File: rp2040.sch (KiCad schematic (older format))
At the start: 29 parts, among them Q5 Q_NMOS_GSD, U17 W25Q128JVS, U3 RP2040, Y2 12MHz

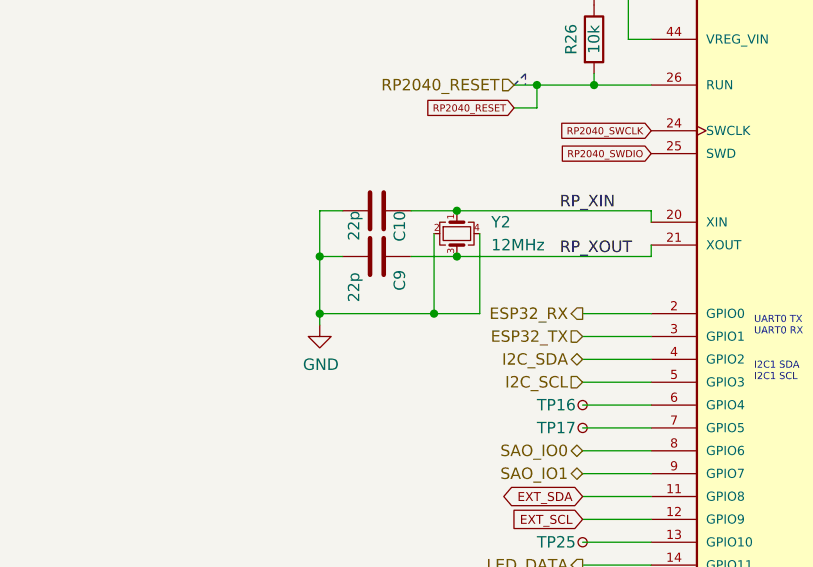
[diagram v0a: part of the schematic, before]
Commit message: Add 1k resistor for RP2040 crystal, add schematic PDF
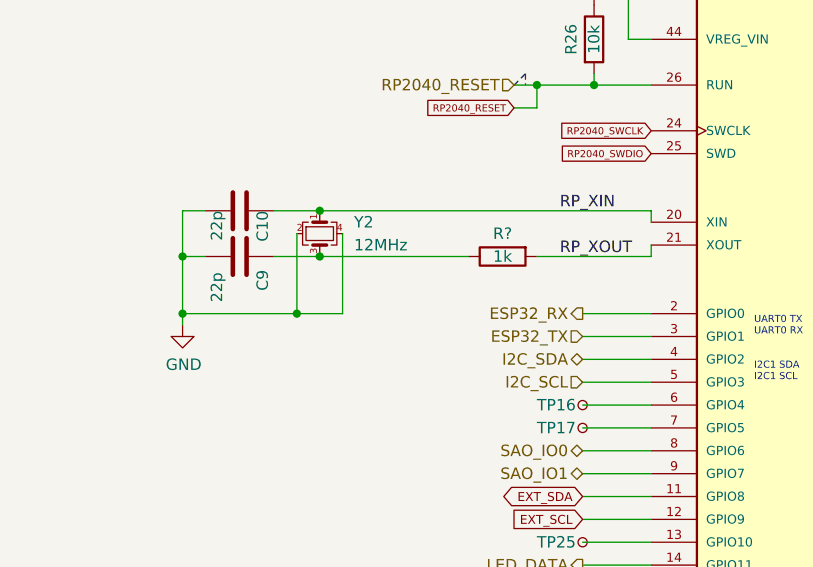
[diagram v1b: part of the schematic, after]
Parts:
- added R?: 1k, Resistor_SMD:R_0402_1005Metric, symbol mch2021-rescue:R-Device
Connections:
- net RP_XOUT: now also R?.2; no longer C9.1, Y2.3
- new net: C9.1, R?.1, Y2.3
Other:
- moved on the sheet: C10, C9, Y2
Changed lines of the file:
@@
 encoding utf-8
 Sheet 3 9
-Title "MCH2021 badge - RP2040 microcontroller"
-Date "2021-11-14"
-Rev "3"
+Title "MCH2022 badge - RP2040 microcontroller"
+Date "2021-12-19"
+Rev "3.1415"
 Comp "BADGE.TEAM"
 Comment1 ""
@@
 L mch2021-rescue:C-Device C?
 U 1 1 5E3EFF6B
-P 3100 3200
+P 2500 3200
 AR Path="/5DC753C3/5E3EFF6B" Ref="C?"  Part="1"
 AR Path="/5E3EFF6B" Ref="C?"  Part="1"
 AR Path="/5E3BA64A/5E3EFF6B" Ref="C?"  Part="1"
 AR Path="/5F51E414/5E3EFF6B" Ref="C10"  Part="1"
-F 0 "C10" H 3100 3300 50  0000 L CNN
-F 1 "22p" H 3100 3100 50  0000 L CNN
-F 2 "Capacitor_SMD:C_0402_1005Metric" H 3138 3050 50  0001 C CNN
-F 3 "" H 3100 3200 50  0001 C CNN
-F 4 "C696906" H 3100 3200 50  0001 C CNN "LCSC"
-F 5 "" H 3100 3200 50  0001 C CNN "Price"
-F 6 "N" H 3100 3200 50  0001 C CNN "Sponsored"
-	1    3100 3200
+F 0 "C10" H 2500 3300 50  0000 L CNN
+F 1 "22p" H 2500 3100 50  0000 L CNN
+F 2 "Capacitor_SMD:C_0402_1005Metric" H 2538 3050 50  0001 C CNN
+F 3 "" H 2500 3200 50  0001 C CNN
+F 4 "C696906" H 2500 3200 50  0001 C CNN "LCSC"
+F 5 "" H 2500 3200 50  0001 C CNN "Price"
+F 6 "N" H 2500 3200 50  0001 C CNN "Sponsored"
+	1    2500 3200
 	0    1    1    0
 $EndComp
@@
 L mch2021-rescue:C-Device C?
 U 1 1 5E3F1F93
-P 3100 3400
+P 2500 3400
 AR Path="/5DC753C3/5E3F1F93" Ref="C?"  Part="1"
 AR Path="/5E3F1F93" Ref="C?"  Part="1"
 AR Path="/5E3BA64A/5E3F1F93" Ref="C?"  Part="1"
 AR Path="/5F51E414/5E3F1F93" Ref="C9"  Part="1"
-F 0 "C9" H 2950 3500 50  0000 L CNN
-F 1 "22p" H 2900 3300 50  0000 L CNN
-F 2 "Capacitor_SMD:C_0402_1005Metric" H 3138 3250 50  0001 C CNN
-F 3 "" H 3100 3400 50  0001 C CNN
-F 4 "C696906" H 3100 3400 50  0001 C CNN "LCSC"
-F 5 "" H 3100 3400 50  0001 C CNN "Price"
-F 6 "N" H 3100 3400 50  0001 C CNN "Sponsored"
-	1    3100 3400
+F 0 "C9" H 2350 3500 50  0000 L CNN
+F 1 "22p" H 2300 3300 50  0000 L CNN
+F 2 "Capacitor_SMD:C_0402_1005Metric" H 2538 3250 50  0001 C CNN
+F 3 "" H 2500 3400 50  0001 C CNN
+F 4 "C696906" H 2500 3400 50  0001 C CNN "LCSC"
+F 5 "" H 2500 3400 50  0001 C CNN "Price"
+F 6 "N" H 2500 3400 50  0001 C CNN "Sponsored"
+	1    2500 3400
 	0    1    -1   0
 $EndComp
@@
 L mch2021-rescue:Crystal_GND24_Small-Device Y2
 U 1 1 5E3ED918
-P 3450 3300
-F 0 "Y2" V 3400 3450 50  0000 L CNN
-F 1 "12MHz" V 3500 3450 50  0000 L CNN
-F 2 "Crystal:Crystal_SMD_3225-4Pin_3.2x2.5mm" H 3450 3300 50  0001 C CNN
-F 3 "~" H 3450 3300 50  0001 C CNN
-F 4 "C13738" H 3450 3300 50  0001 C CNN "LCSC"
-F 5 "" H 3450 3300 50  0001 C CNN "Price"
-F 6 "-" H 3450 3300 50  0001 C CNN "Mouser"
-F 7 "N" H 3450 3300 50  0001 C CNN "Sponsored"
-	1    3450 3300
+P 2850 3300
+F 0 "Y2" V 2800 3450 50  0000 L CNN
+F 1 "12MHz" V 2900 3450 50  0000 L CNN
+F 2 "Crystal:Crystal_SMD_3225-4Pin_3.2x2.5mm" H 2850 3300 50  0001 C CNN
+F 3 "~" H 2850 3300 50  0001 C CNN
+F 4 "C13738" H 2850 3300 50  0001 C CNN "LCSC"
+F 5 "" H 2850 3300 50  0001 C CNN "Price"
+F 6 "-" H 2850 3300 50  0001 C CNN "Mouser"
+F 7 "N" H 2850 3300 50  0001 C CNN "Sponsored"
+	1    2850 3300
 	0    1    1    0
 $EndComp
@@
 L mch2021-rescue:GND-power #PWR051
 U 1 1 5F916F4B
-P 2850 3700
-F 0 "#PWR051" H 2850 3450 50  0001 C CNN
-F 1 "GND" H 2855 3527 50  0000 C CNN
-F 2 "" H 2850 3700 50  0001 C CNN
-F 3 "" H 2850 3700 50  0001 C CNN
-	1    2850 3700
+P 2250 3700
+F 0 "#PWR051" H 2250 3450 50  0001 C CNN
+F 1 "GND" H 2255 3527 50  0000 C CNN
+F 2 "" H 2250 3700 50  0001 C CNN
+F 3 "" H 2250 3700 50  0001 C CNN
+	1    2250 3700
 	1    0    0    -1
 $EndComp
@@
 	6100 4850 6450 4850
 Wire Wire Line
-	3450 3400 3250 3400
-Connection ~ 3450 3400
-Wire Wire Line
-	3450 3200 3250 3200
-Connection ~ 3450 3200
+	2850 3400 2650 3400
+Wire Wire Line
+	2850 3200 2650 3200
+Connection ~ 2850 3200
 Wire Wire Line
 	4300 3400 4300 3350
 Wire Wire Line
-	3450 3400 4300 3400
-Wire Wire Line
 	4300 3200 4300 3250
 Wire Wire Line
-	3450 3200 4300 3200
-Wire Wire Line
-	2850 3700 2850 3650
-Wire Wire Line
-	2850 3200 2950 3200
-Wire Wire Line
-	2950 3400 2850 3400
-Connection ~ 2850 3400
-Wire Wire Line
-	2850 3400 2850 3200
-Connection ~ 2850 3650
-Wire Wire Line
-	2850 3650 2850 3400
+	2250 3700 2250 3650
+Wire Wire Line
+	2250 3200 2350 3200
+Wire Wire Line
+	2350 3400 2250 3400
+Connection ~ 2250 3400
+Wire Wire Line
+	2250 3400 2250 3200
+Connection ~ 2250 3650
+Wire Wire Line
+	2250 3650 2250 3400
 Wire Wire Line
 	7150 4250 7050 4250
@@
 $EndComp
 Wire Wire Line
-	3550 3300 3550 3650
-Wire Wire Line
-	3350 3650 3350 3300
-Connection ~ 3350 3650
-Wire Wire Line
-	3350 3650 3550 3650
-Wire Wire Line
-	2850 3650 3350 3650
+	2950 3300 2950 3650
+Wire Wire Line
+	2750 3650 2750 3300
+Connection ~ 2750 3650
+Wire Wire Line
+	2750 3650 2950 3650
+Wire Wire Line
+	2250 3650 2750 3650
 Wire Wire Line
 	4000 3650 4300 3650
@@
 	1    0    0    -1
 $EndComp
+Wire Wire Line
+	2850 3200 4300 3200
+$Comp
+L mch2021-rescue:R-Device R?
+U 1 1 61C35D5C
+P 3650 3400
+AR Path="/5DC753C3/61C35D5C" Ref="R?"  Part="1"
+AR Path="/61C35D5C" Ref="R?"  Part="1"
+AR Path="/5E3BA64A/61C35D5C" Ref="R?"  Part="1"
+AR Path="/5F51E414/61C35D5C" Ref="R?"  Part="1"
+AR Path="/5FDC6C76/61C35D5C" Ref="R?"  Part="1"
+F 0 "R?" V 3550 3400 50  0000 C CNN
+F 1 "1k" V 3650 3400 50  0000 C CNN
+F 2 "Resistor_SMD:R_0402_1005Metric" V 3580 3400 50  0001 C CNN
+F 3 "~" H 3650 3400 50  0001 C CNN
+F 4 "" H 3650 3400 50  0001 C CNN "LCSC"
+F 5 "" H 3650 3400 50  0001 C CNN "Price"
+F 6 "-" H 3650 3400 50  0001 C CNN "Mouser"
+F 7 "N" H 3650 3400 50  0001 C CNN "Sponsored"
+	1    3650 3400
+	0    -1   1    0
+$EndComp
+Wire Wire Line
+	3800 3400 4300 3400
+Wire Wire Line
+	3500 3400 2850 3400
+Connection ~ 2850 3400
 $EndSCHEMATC
